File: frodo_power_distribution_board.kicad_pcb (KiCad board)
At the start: 2 copper layers, 27 parts, among them J1 Payload_1, J2 Payload_2, J3 Payload_3, J4 Conn_01x06, J5 Conn_01x06

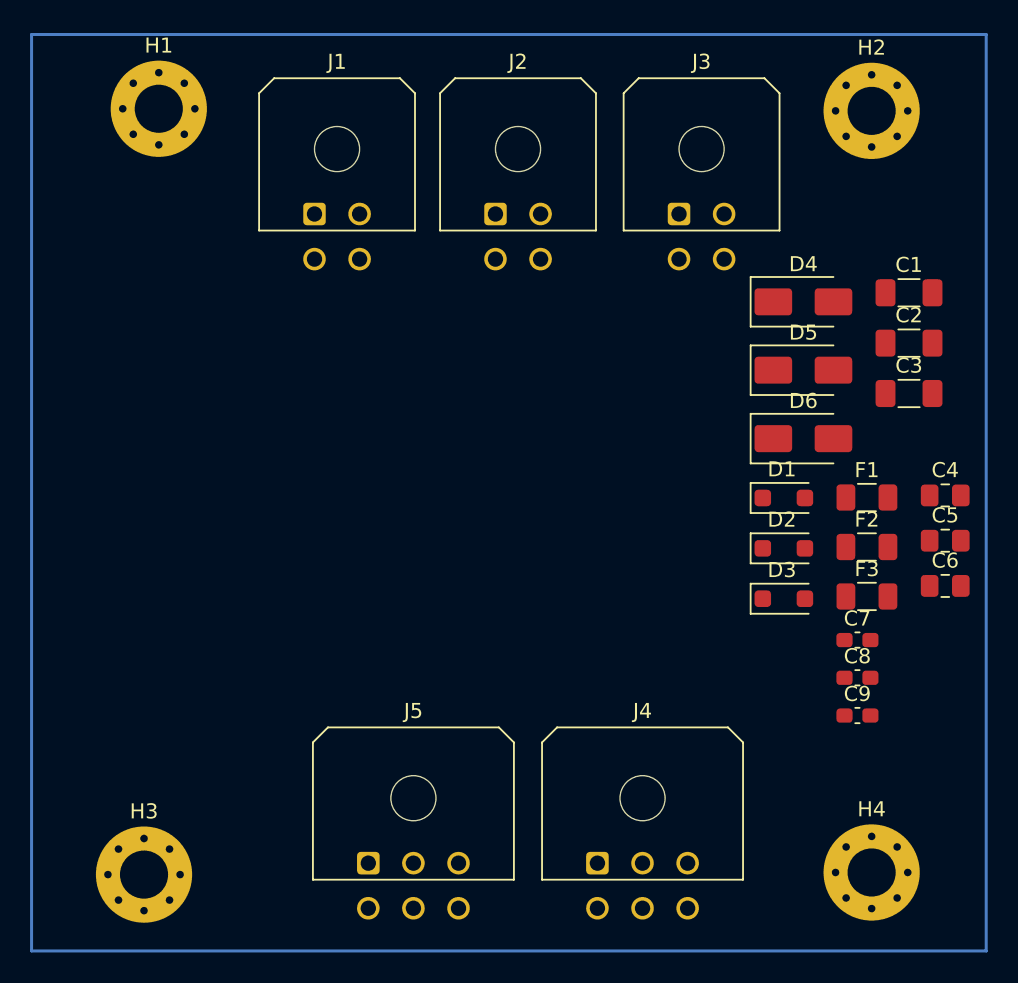
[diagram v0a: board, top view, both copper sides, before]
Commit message: First iteration of board layout
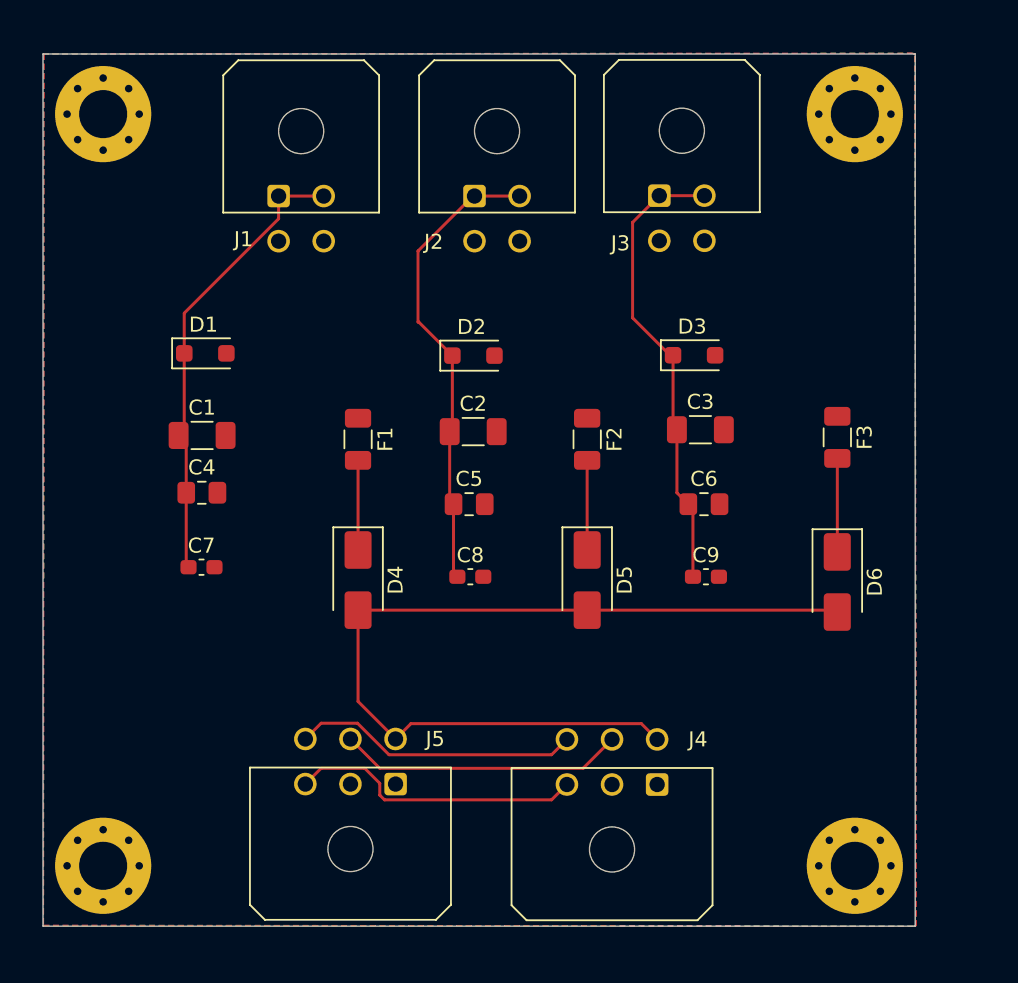
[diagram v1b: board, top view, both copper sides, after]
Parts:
- moved C4 49.5 mm to (92.6, 96.5)
- moved C1 48.0 mm to (92.6, 92.7)
- moved C7 43.9 mm to (92.6, 101.5)
- moved D1 39.7 mm to (92.8, 87.2)
- moved D4 34.9 mm to (103.0, 102.3), turned to -90 degrees
- moved F1 34.1 mm to (103.0, 93.0), turned to -90 degrees
- moved C5 31.8 mm to (110.4, 97.3)
- moved C2 29.6 mm to (110.7, 92.5)
- moved C8 26.6 mm to (110.5, 102.1)
- moved D2 24.3 mm to (110.7, 87.4)
- moved D5 20.0 mm to (118.2, 102.3), turned to -90 degrees
- moved F2 19.9 mm to (118.2, 93.0), turned to -90 degrees
- moved D3 17.3 mm to (125.3, 87.4)
- moved C6 16.9 mm to (126.0, 97.3)
- moved C3 14.1 mm to (125.8, 92.3)
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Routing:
- net VDC: track 0.00 -> 59.8 mm
- net Net-(D2-K): track 0.00 -> 31.2 mm
- net Net-(D3-K): track 0.00 -> 30.9 mm
- net Net-(D1-K): track 0.00 -> 30.7 mm
- net CAN-: track 0.00 -> 19.6 mm
- net CAN+: track 0.00 -> 19.1 mm
- net Net-(J4-Pin_5): track 0.00 -> 19.0 mm
- net Net-(D6-K): track 0.00 -> 6.22 mm
- net Net-(D5-K): track 0.00 -> 5.96 mm
- net Net-(D4-K): track 0.00 -> 5.96 mm
- added copper zone on B.Cu, net GND
- added copper zone on F.Cu, net GND
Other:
- board outline added: 58 x 58 mm
